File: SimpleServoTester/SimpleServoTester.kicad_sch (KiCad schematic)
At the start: 8 parts, among them SW1 POWER, U1 ATmega328-A, U2 L7805

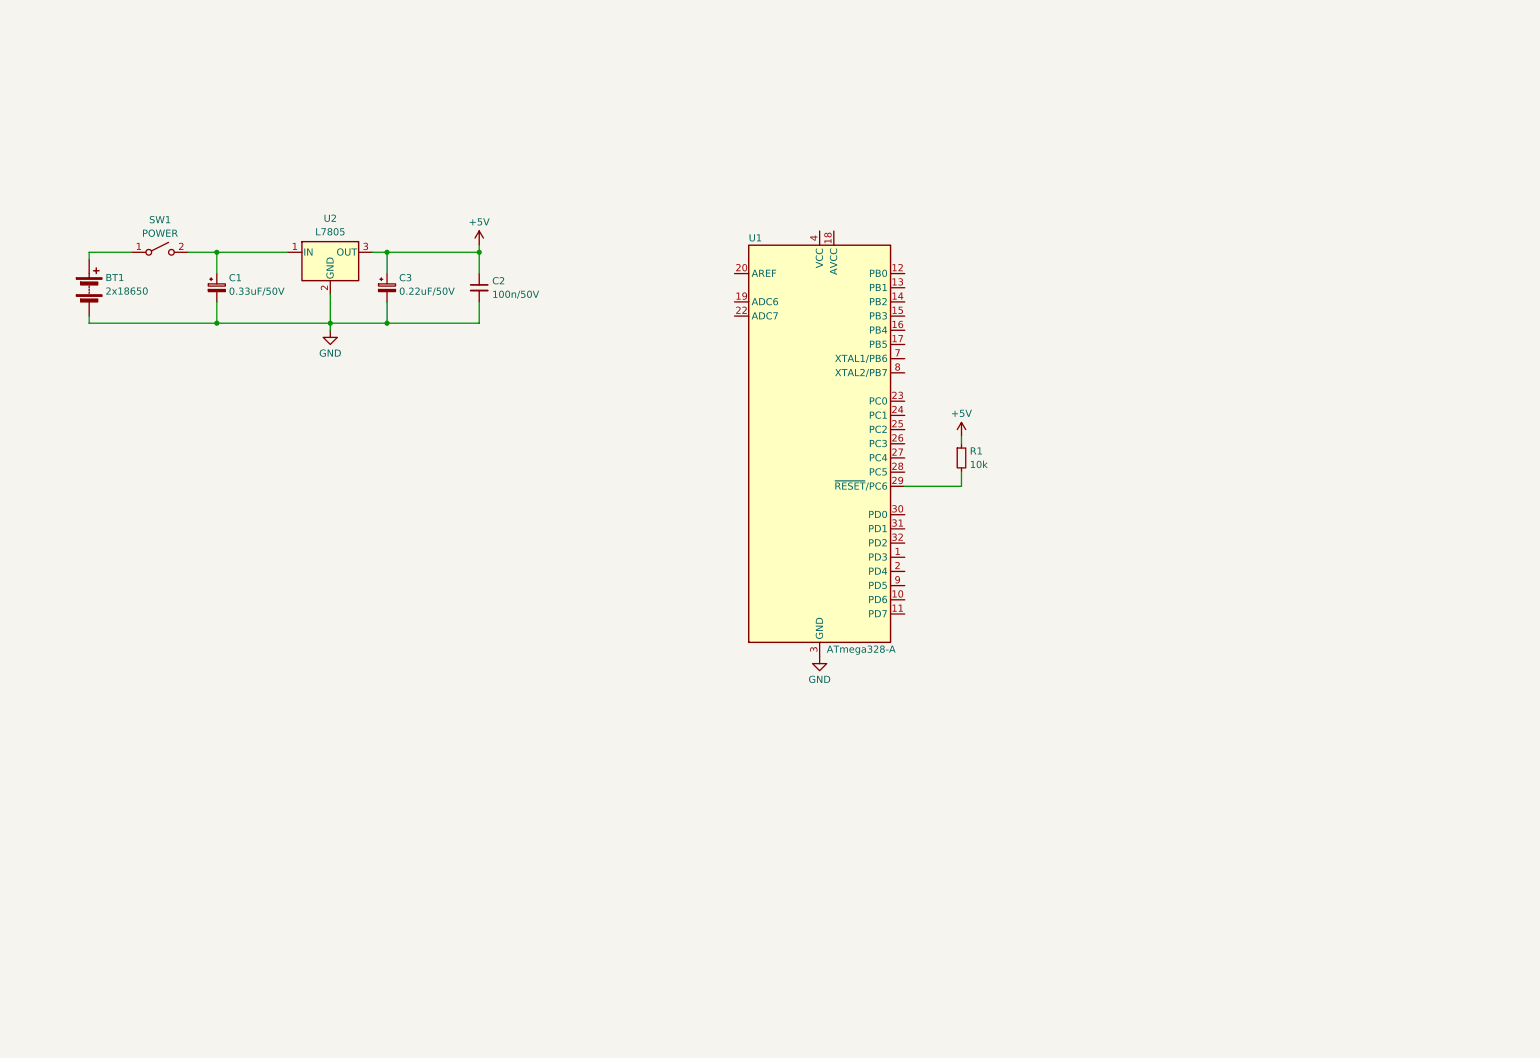
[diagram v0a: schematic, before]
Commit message: update
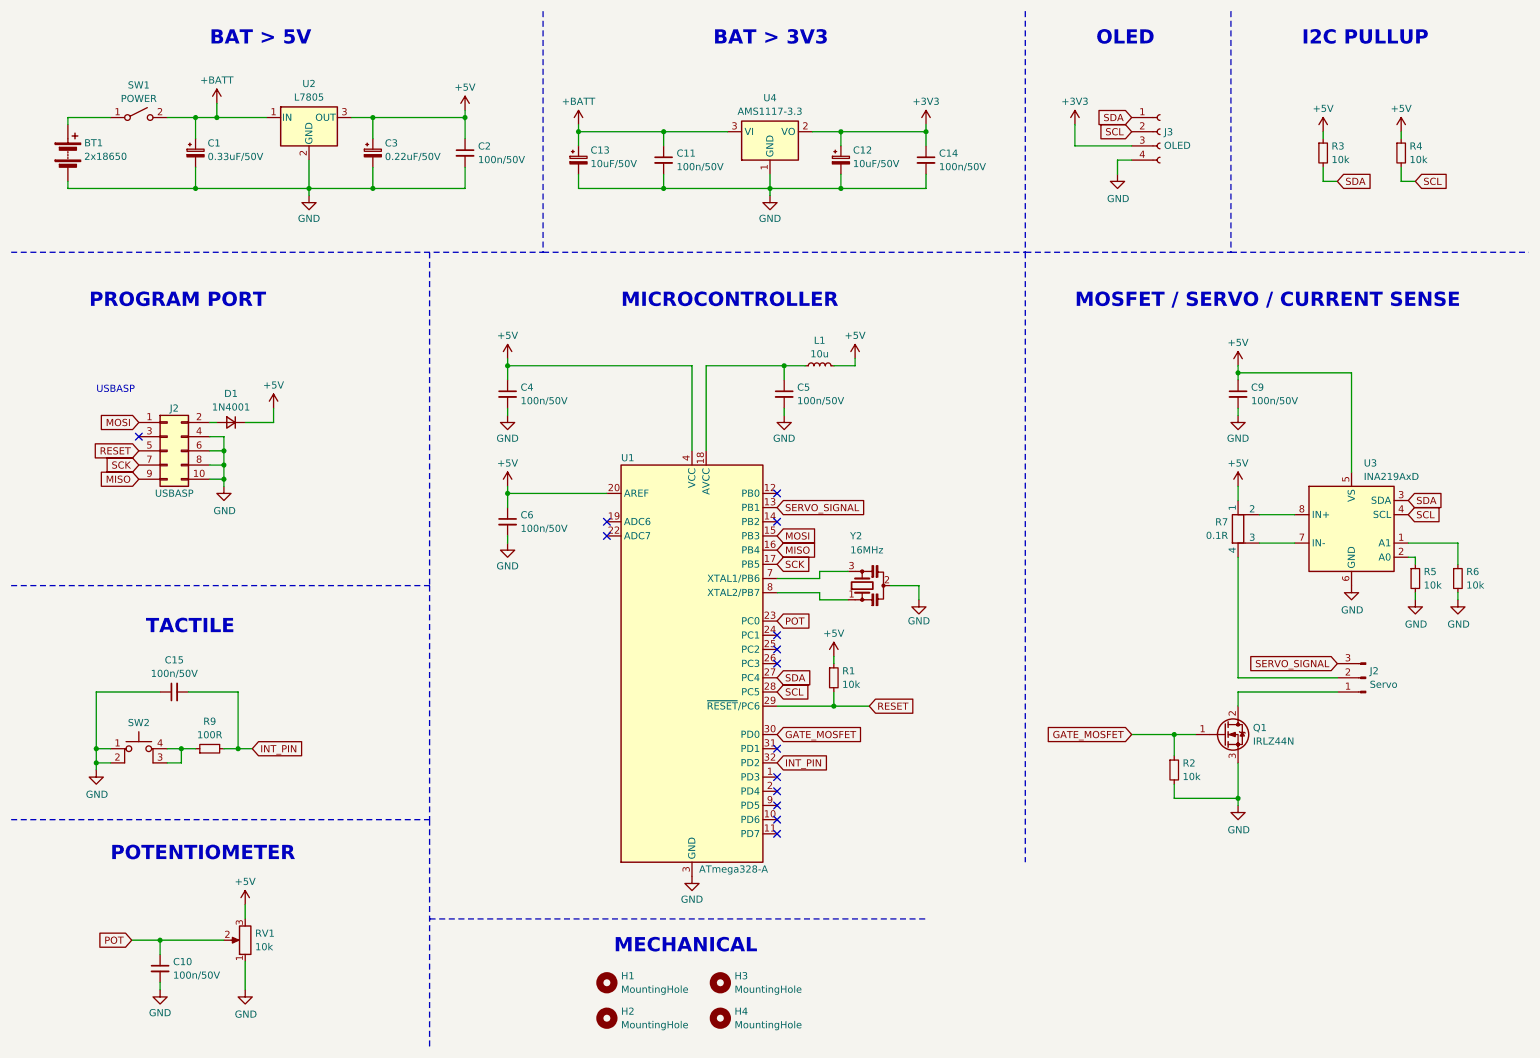
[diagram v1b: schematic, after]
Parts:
- added C10, C11, C14, C15, C4, C5, C6, C9: 100n/50V, symbol Device:C_Small
- added C12, C13: 10uF/50V, symbol Device:C_Polarized_Small
- added D1: 1N4001, symbol Device:D_Small
- added H1, H2, H3, H4: MountingHole, symbol Mechanical:MountingHole
- added J2: Servo, symbol Connector:Conn_01x03_Pin
- added J2: USBASP, Connector_IDC:IDC-Header_2x05_P2.54mm_Horizontal, symbol Connector_Generic:Conn_02x05_Odd_Even
- added J3: OLED, symbol Connector:Conn_01x04_Socket
- added L1: 10u, symbol Device:L_Small
- added Q1: IRLZ44N, Package_TO_SOT_THT:TO-220-3_Vertical, symbol Transistor_FET:IRLZ44N
- added R2, R3, R4, R5, R6: 10k, symbol Device:R_Small
- added R7: 0.1R, symbol Device:R_Shunt
- added R9: 100R, symbol Device:R_Small
- added RV1: 10k, symbol Device:R_Potentiometer
- added SW2: Tactile, symbol Switch:SW_MEC_5E
- added U3: INA219AxD, Package_SO:SOIC-8_3.9x4.9mm_P1.27mm, symbol Sensor_Energy:INA219AxD
- added U4: AMS1117-3.3, Package_TO_SOT_SMD:SOT-223-3_TabPin2, symbol Regulator_Linear:AMS1117-3.3
- added Y2: 16MHz, Footprint:CSTCE16M0V53-R0, symbol Device:Resonator_Small
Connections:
- net +5V: now also U1.20 (AREF), U1.4 (VCC), U1.6 (VCC), C4.1, C6.1, C9.1, D1.1 (K), L1.2, R3.1, R4.1, R7.1, RV1.3, U3.5 (VS)
- net GND: now also C10.2, C11.2, C12.2, C13.2, C14.2, C15.1, C4.2, C5.2, C6.2, C9.2, J2.10 (Pin_10), J2.4 (Pin_4), J2.6 (Pin_6), J2.8 (Pin_8), J3.4 (Pin_4), Q1.3 (S), R2.2, R5.2, R6.2, RV1.1, SW2.1, SW2.2, U3.6 (GND), U4.1 (GND), Y2.2
- net +BATT: now reaches C1.1, SW1.2 (B), U2.1 (IN)
- net +BATT: now also C11.1, C13.1, U4.3 (VI)
- net SERVO_SIGNAL: now reaches U1.13 (PB1)
- net SERVO_SIGNAL: now also J2.3 (Pin_3)
- net MOSI: now reaches U1.15 (PB3)
- net MOSI: now also J2.1 (Pin_1)
- net MISO: now reaches U1.16 (PB4)
- net MISO: now also J2.9 (Pin_9)
- net SCK: now reaches U1.17 (PB5)
- net SCK: now also J2.7 (Pin_7)
- net at U1.18 (AVCC): now also C5.1, L1.1
- net POT: now reaches U1.23 (PC0)
- net POT: now also C10.1, RV1.2
- net SDA: now reaches U1.27 (PC4)
- net SDA: now also J3.1 (Pin_1), R3.2, U3.3 (SDA)
- net SCL: now reaches U1.28 (PC5)
- net SCL: now also J3.2 (Pin_2), R4.2, U3.4 (SCL)
- net RESET: now reaches R1.2, U1.29 (~{RESET}/PC6)
- net RESET: now also J2.5 (Pin_5)
- net GATE_MOSFET: now reaches U1.30 (PD0)
- net GATE_MOSFET: now also Q1.1 (G), R2.1
- net INT_PIN: now reaches U1.32 (PD2)
- net INT_PIN: now also C15.2, R9.2
- net at U1.7 (XTAL1/PB6): now also Y2.3
- net at U1.8 (XTAL2/PB7): now also Y2.1
- new net: R6.1, U3.1 (A1)
- new net: J2.1 (Pin_1), Q1.2 (D)
- new net: D1.2 (A), J2.2 (Pin_2)
- new net: J2.2 (Pin_2), R7.4
- new net: R9.1, SW2.3 (K), SW2.4 (A)
- new net: R5.1, U3.2 (A0)
- new net: R7.3, U3.7 (IN-)
- new net: R7.2, U3.8 (IN+)
- new net +3V3: C12.1, C14.1, J3.3 (Pin_3), U4.2 (VO)
- no-connect marks 0 -> 14
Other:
- note added: "BAT > 3V3"
- note added: "BAT > 5V"
- note added: "I2C PULLUP"
- note added: "MECHANICAL"
- note added: "MICROCONTROLLER"
- note added: "MOSFET / SERVO / CURRENT SENSE"
- note added: "OLED"
- note added: "POTENTIOMETER"
- note added: "PROGRAM PORT"
- note added: "TACTILE"
- note added: "USBASP"
- moved on the sheet: BT1, C1, C2, C3, R1, SW1, U1, U2
